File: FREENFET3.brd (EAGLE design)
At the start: 35.6 x 17.8 mm, 24 parts, among them IC1 WS2811-SOP8, J1 IN, J2 OUT, Q1 NTD5867NLT4G, Q2 NTD5867NLT4G, Q3 NTD5867NLT4G, Q4 MOSFET-NSOT-323, Q5 MOSFET-NSOT-323, Q6 MOSFET-NSOT-323

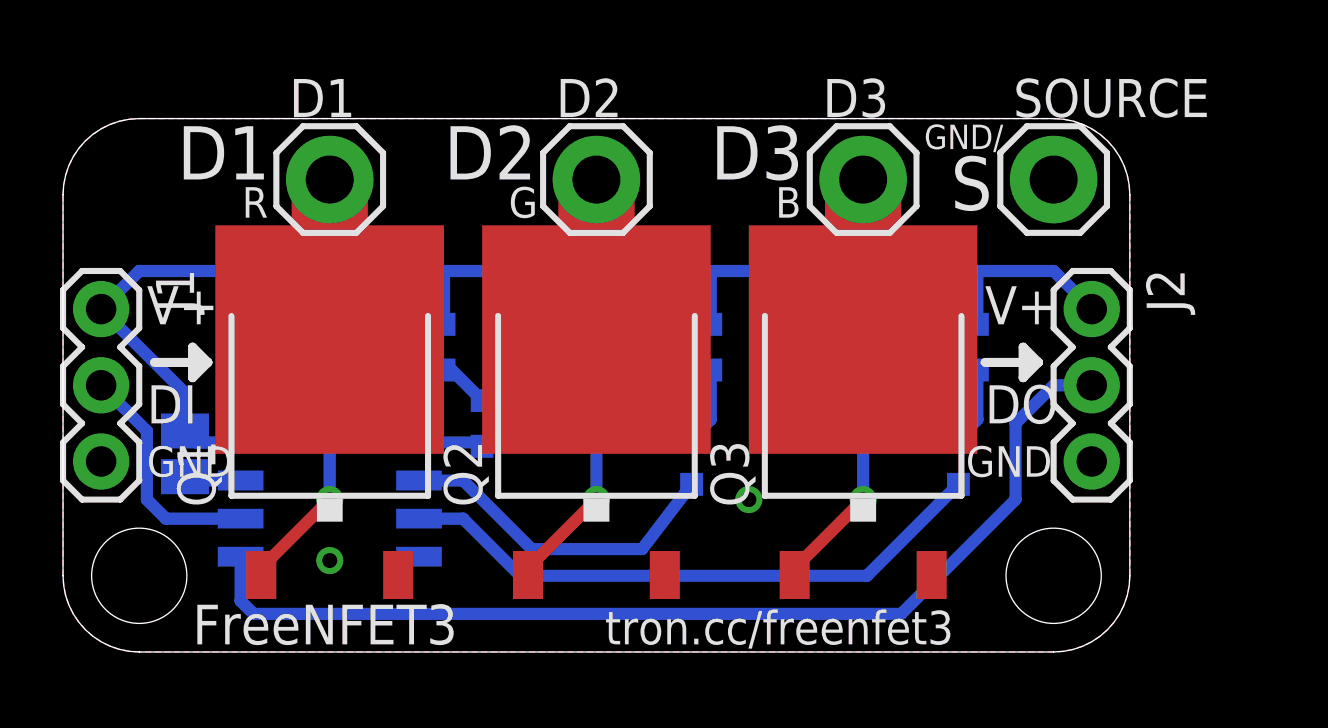
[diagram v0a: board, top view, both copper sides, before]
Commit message: Final layout
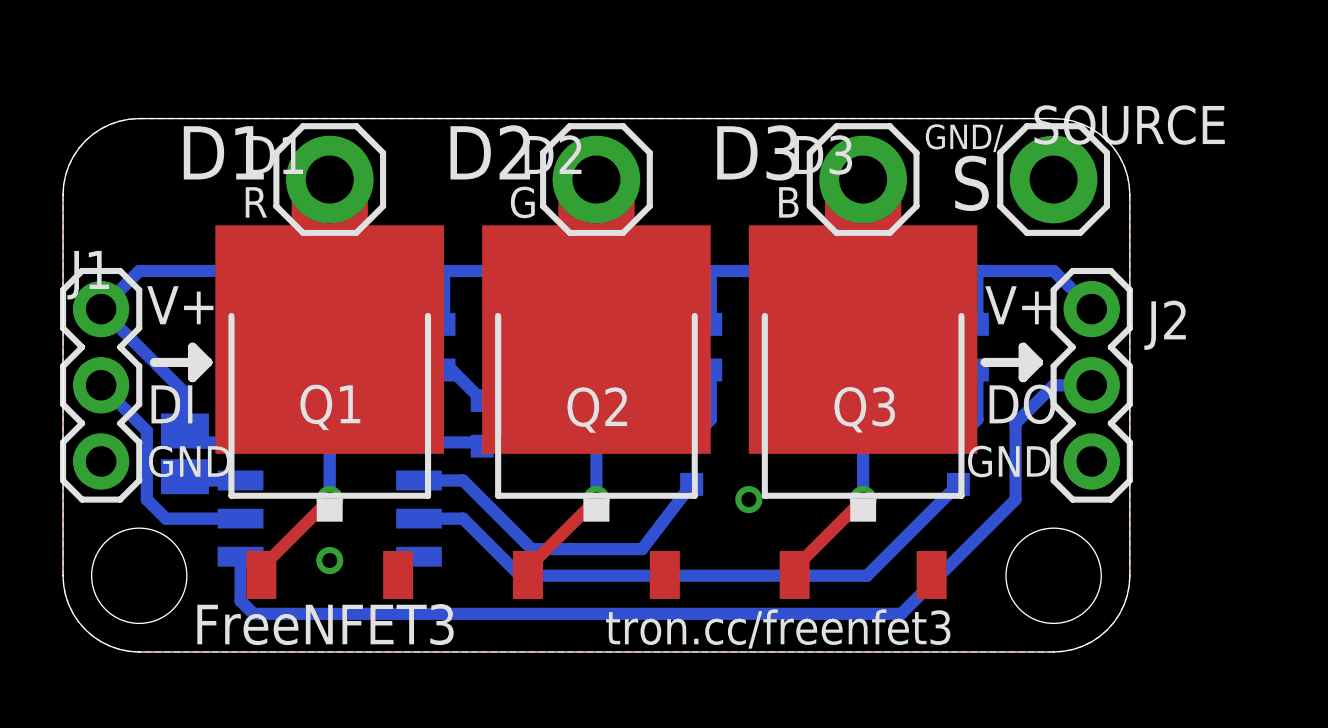
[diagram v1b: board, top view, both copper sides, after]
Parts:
- Q4, Q5, Q6: value MOSFET-NSOT-323 -> RJU003N03
